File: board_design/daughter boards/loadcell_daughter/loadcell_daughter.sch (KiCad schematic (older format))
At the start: 8 parts, among them J1 Conn_01x09_Male, J2 Conn_01x04, U1 AD8613, U2 AD8227

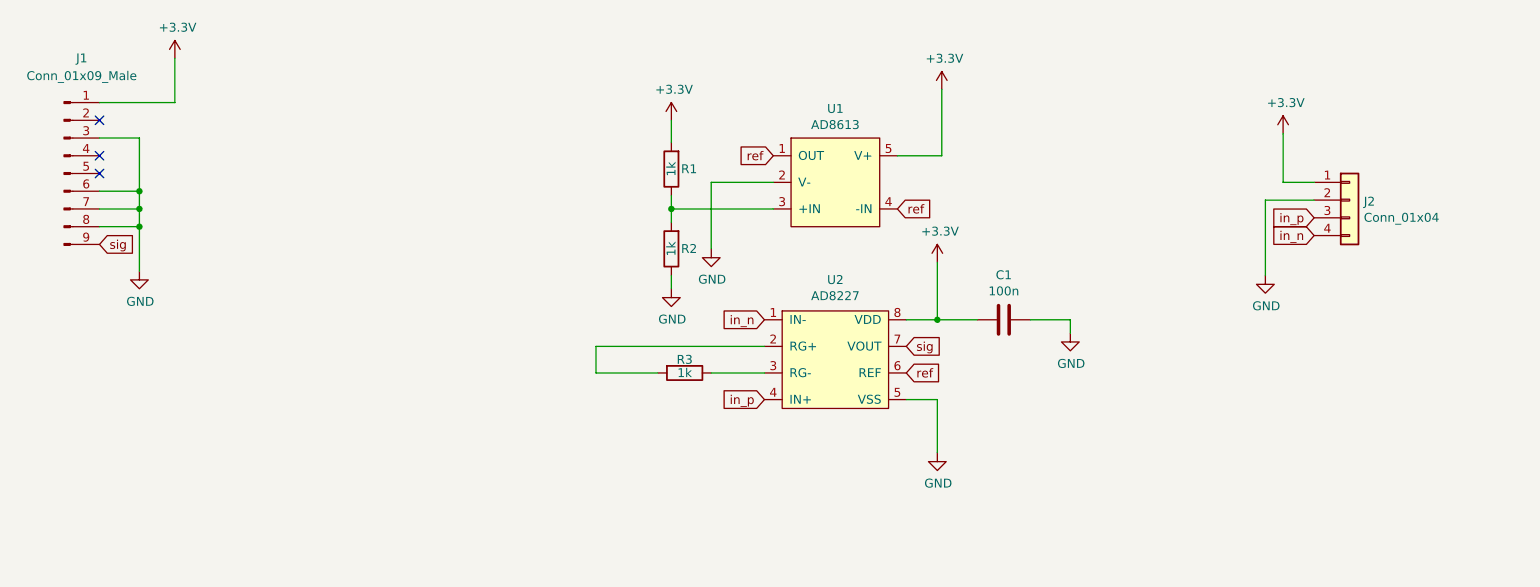
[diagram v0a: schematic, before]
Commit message: first MX export
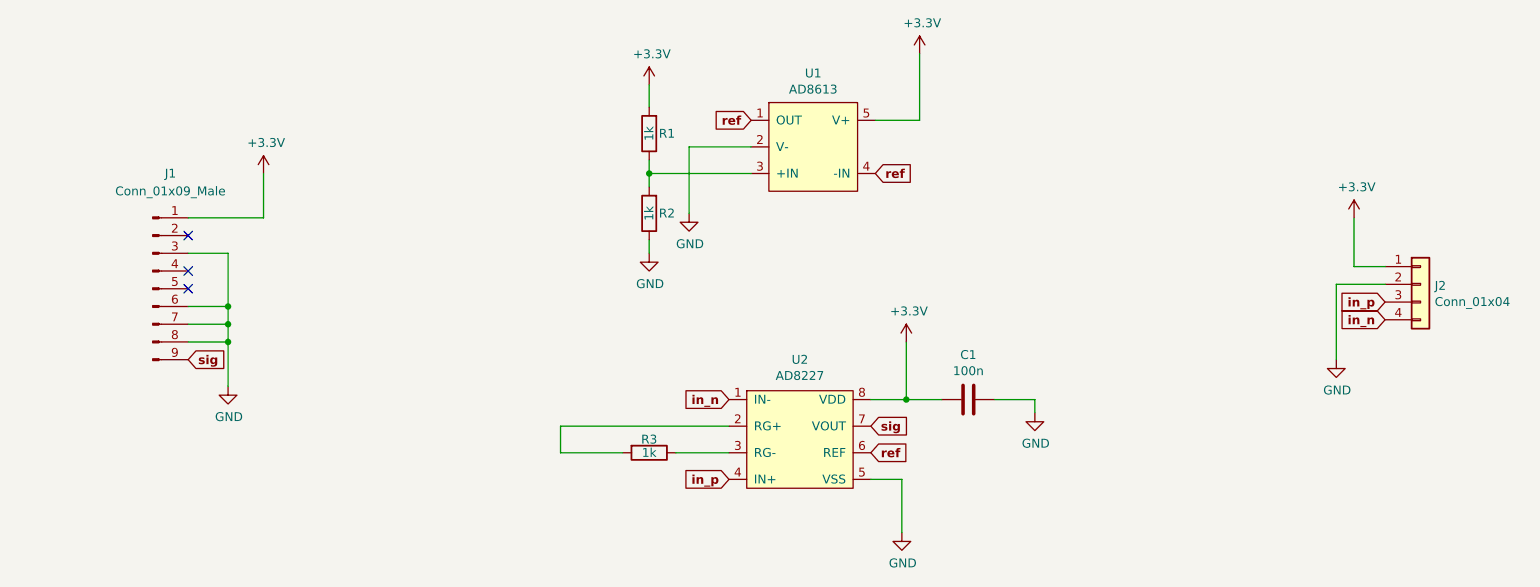
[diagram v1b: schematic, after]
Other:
- moved on the sheet: C1, J1, J2, R1, R2, R3, U1, U2
